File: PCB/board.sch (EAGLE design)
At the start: 33 parts, among them IC2 LM340MP-05, J1 DCJ0202, J2 DCJ0202, Q1 CRYSTAL_16MHZ_SMD, U1 MLX90614_, U2 MMA8451

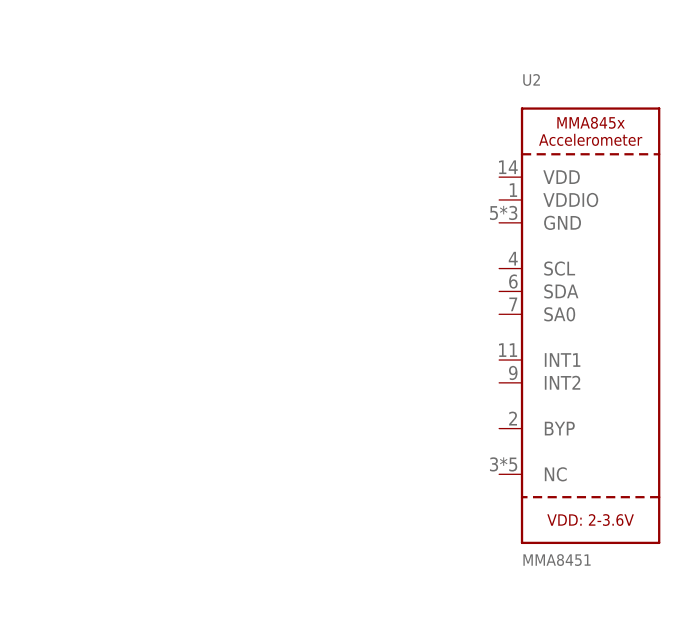
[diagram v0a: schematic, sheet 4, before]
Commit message: Nothing
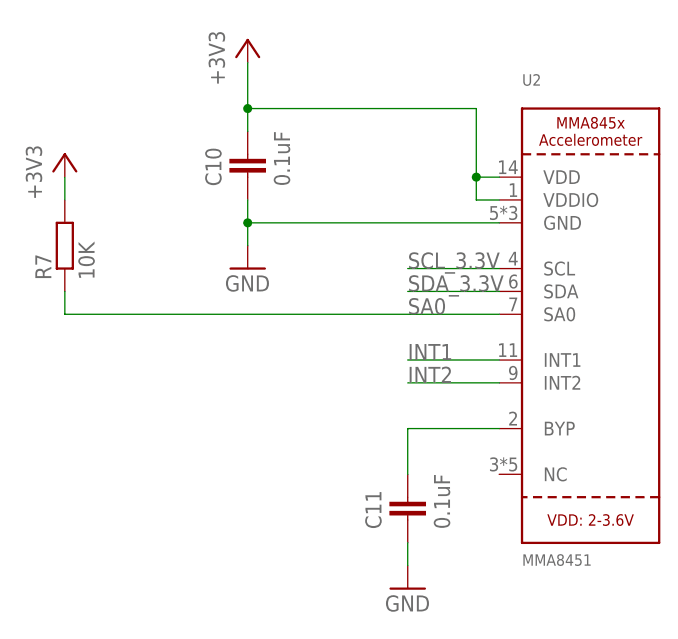
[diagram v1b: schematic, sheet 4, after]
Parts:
- added C10, C11: 0.1uF, rcl:C-EUC0805
- added R7: 10K, rcl:R-EU_R0805
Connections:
- new net INT1: U2.INT1
- new net INT2: U2.INT2
- new net N$40: C11.1, U2.BYP
- new net SA0: R7.1, U2.SA0
- new net SCL_3.3V: U2.SCL
- new net SDA_3.3V: U2.SDA
- net +3V3: now also C10.1, R7.2, U2.VDD, U2.VDDIO
- net GND: now also C10.2, C11.2, U2.GND
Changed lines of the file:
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@@
 <?xml version="1.0" encoding="utf-8"?>
 <!DOCTYPE eagle SYSTEM "eagle.dtd">
-<eagle version="9.4.2">
+<eagle version="9.5.1">
 <drawing>
 <settings>
-<setting alwaysvectorfont="no"/>
+<setting alwaysvectorfont="yes"/>
 <setting verticaltext="up"/>
 </settings>
@@
 <part name="+3V4" library="supply1" library_urn="urn:adsk.eagle:library:371" deviceset="+3V3" device=""/>
 <part name="U2" library="microbuilder" deviceset="ACCEL_MMA845X" device="" value="MMA8451"/>
+<part name="+3V5" library="supply1" library_urn="urn:adsk.eagle:library:371" deviceset="+3V3" device=""/>
+<part name="C10" library="rcl" library_urn="urn:adsk.eagle:library:334" deviceset="C-EU" device="C0805" package3d_urn="urn:adsk.eagle:package:23617/2" value="0.1uF"/>
+<part name="GND16" library="supply1" library_urn="urn:adsk.eagle:library:371" deviceset="GND" device=""/>
+<part name="R7" library="rcl" library_urn="urn:adsk.eagle:library:334" deviceset="R-EU_" device="R0805" package3d_urn="urn:adsk.eagle:package:23553/2" value="10K"/>
+<part name="+3V6" library="supply1" library_urn="urn:adsk.eagle:library:371" deviceset="+3V3" device=""/>
+<part name="C11" library="rcl" library_urn="urn:adsk.eagle:library:334" deviceset="C-EU" device="C0805" package3d_urn="urn:adsk.eagle:package:23617/2" value="0.1uF"/>
+<part name="GND17" library="supply1" library_urn="urn:adsk.eagle:library:371" deviceset="GND" device=""/>
 </parts>
 <sheets>
@@
 <attribute name="VALUE" x="73.66" y="25.4" size="1.27" layer="96"/>
 </instance>
+<instance part="+3V5" gate="G$1" x="43.18" y="83.82" smashed="yes">
+<attribute name="VALUE" x="40.64" y="78.74" size="1.778" layer="96" rot="R90"/>
+</instance>
+<instance part="C10" gate="G$1" x="43.18" y="71.12" smashed="yes">
+<attribute name="NAME" x="40.259" y="67.564" size="1.778" layer="95" rot="R90"/>
+<attribute name="VALUE" x="47.879" y="67.564" size="1.778" layer="96" rot="R90"/>
+</instance>
+<instance part="GND16" gate="1" x="43.18" y="58.42" smashed="yes">
+<attribute name="VALUE" x="40.64" y="55.88" size="1.778" layer="96"/>
+</instance>
+<instance part="R7" gate="G$1" x="22.86" y="60.96" smashed="yes" rot="R90">
+<attribute name="NAME" x="21.3614" y="57.15" size="1.778" layer="95" rot="R90"/>
+<attribute name="VALUE" x="26.162" y="57.15" size="1.778" layer="96" rot="R90"/>
+</instance>
+<instance part="+3V6" gate="G$1" x="22.86" y="71.12" smashed="yes">
+<attribute name="VALUE" x="20.32" y="66.04" size="1.778" layer="96" rot="R90"/>
+</instance>
+<instance part="C11" gate="G$1" x="60.96" y="33.02" smashed="yes">
+<attribute name="NAME" x="58.039" y="29.464" size="1.778" layer="95" rot="R90"/>
+<attribute name="VALUE" x="65.659" y="29.464" size="1.778" layer="96" rot="R90"/>
+</instance>
+<instance part="GND17" gate="1" x="60.96" y="22.86" smashed="yes">
+<attribute name="VALUE" x="58.42" y="20.32" size="1.778" layer="96"/>
+</instance>
 </instances>
 <busses>
 </busses>
 <nets>
+<net name="+3V3" class="0">
+<segment>
+<pinref part="U2" gate="G$1" pin="VDDIO"/>
+<wire x1="71.12" y1="66.04" x2="68.58" y2="66.04" width="0.1524" layer="91"/>
+<wire x1="68.58" y1="66.04" x2="68.58" y2="68.58" width="0.1524" layer="91"/>
+<pinref part="U2" gate="G$1" pin="VDD"/>
+<wire x1="68.58" y1="68.58" x2="71.12" y2="68.58" width="0.1524" layer="91"/>
+<wire x1="68.58" y1="68.58" x2="68.58" y2="76.2" width="0.1524" layer="91"/>
+<junction x="68.58" y="68.58"/>
+<wire x1="68.58" y1="76.2" x2="43.18" y2="76.2" width="0.1524" layer="91"/>
+<pinref part="+3V5" gate="G$1" pin="+3V3"/>
+<wire x1="43.18" y1="76.2" x2="43.18" y2="81.28" width="0.1524" layer="91"/>
+<pinref part="C10" gate="G$1" pin="1"/>
+<wire x1="43.18" y1="76.2" x2="43.18" y2="73.66" width="0.1524" layer="91"/>
+<junction x="43.18" y="76.2"/>
+</segment>
+<segment>
+<pinref part="+3V6" gate="G$1" pin="+3V3"/>
+<pinref part="R7" gate="G$1" pin="2"/>
+<wire x1="22.86" y1="68.58" x2="22.86" y2="66.04" width="0.1524" layer="91"/>
+</segment>
+</net>
+<net name="GND" class="0">
+<segment>
+<pinref part="C10" gate="G$1" pin="2"/>
+<wire x1="43.18" y1="66.04" x2="43.18" y2="63.5" width="0.1524" layer="91"/>
+<pinref part="U2" gate="G$1" pin="GND"/>
+<wire x1="43.18" y1="63.5" x2="71.12" y2="63.5" width="0.1524" layer="91"/>
+<wire x1="43.18" y1="63.5" x2="43.18" y2="60.96" width="0.1524" layer="91"/>
+<junction x="43.18" y="63.5"/>
+<pinref part="GND16" gate="1" pin="GND"/>
+</segment>
+<segment>
+<pinref part="GND17" gate="1" pin="GND"/>
+<pinref part="C11" gate="G$1" pin="2"/>
+<wire x1="60.96" y1="25.4" x2="60.96" y2="27.94" width="0.1524" layer="91"/>
+</segment>
+</net>
+<net name="SCL_3.3V" class="0">
+<segment>
+<pinref part="U2" gate="G$1" pin="SCL"/>
+<wire x1="71.12" y1="58.42" x2="60.96" y2="58.42" width="0.1524" layer="91"/>
+<label x="60.96" y="58.42" size="1.778" layer="95"/>
+</segment>
+</net>
+<net name="SDA_3.3V" class="0">
+<segment>
+<pinref part="U2" gate="G$1" pin="SDA"/>
+<wire x1="71.12" y1="55.88" x2="60.96" y2="55.88" width="0.1524" layer="91"/>
+<label x="60.96" y="55.88" size="1.778" layer="95"/>
+</segment>
+</net>
+<net name="SA0" class="0">
+<segment>
+<pinref part="U2" gate="G$1" pin="SA0"/>
+<wire x1="71.12" y1="53.34" x2="22.86" y2="53.34" width="0.1524" layer="91"/>
+<wire x1="22.86" y1="53.34" x2="22.86" y2="55.88" width="0.1524" layer="91"/>
+<label x="60.96" y="53.34" size="1.778" layer="95"/>
+<pinref part="R7" gate="G$1" pin="1"/>
+</segment>
+</net>
+<net name="INT1" class="0">
+<segment>
+<pinref part="U2" gate="G$1" pin="INT1"/>
+<wire x1="71.12" y1="48.26" x2="60.96" y2="48.26" width="0.1524" layer="91"/>
+<label x="60.96" y="48.26" size="1.778" layer="95"/>
+</segment>
+</net>
+<net name="INT2" class="0">
+<segment>
+<pinref part="U2" gate="G$1" pin="INT2"/>
+<wire x1="71.12" y1="45.72" x2="60.96" y2="45.72" width="0.1524" layer="91"/>
+<label x="60.96" y="45.72" size="1.778" layer="95"/>
+</segment>
+</net>
+<net name="N$40" class="0">
+<segment>
+<pinref part="U2" gate="G$1" pin="BYP"/>
+<wire x1="71.12" y1="40.64" x2="60.96" y2="40.64" width="0.1524" layer="91"/>
+<wire x1="60.96" y1="40.64" x2="60.96" y2="35.56" width="0.1524" layer="91"/>
+<pinref part="C11" gate="G$1" pin="1"/>
+</segment>
+</net>
 </nets>
 </sheet>
